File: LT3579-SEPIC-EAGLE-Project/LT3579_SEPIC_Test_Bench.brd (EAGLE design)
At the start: 74 x 58 mm, 160 parts

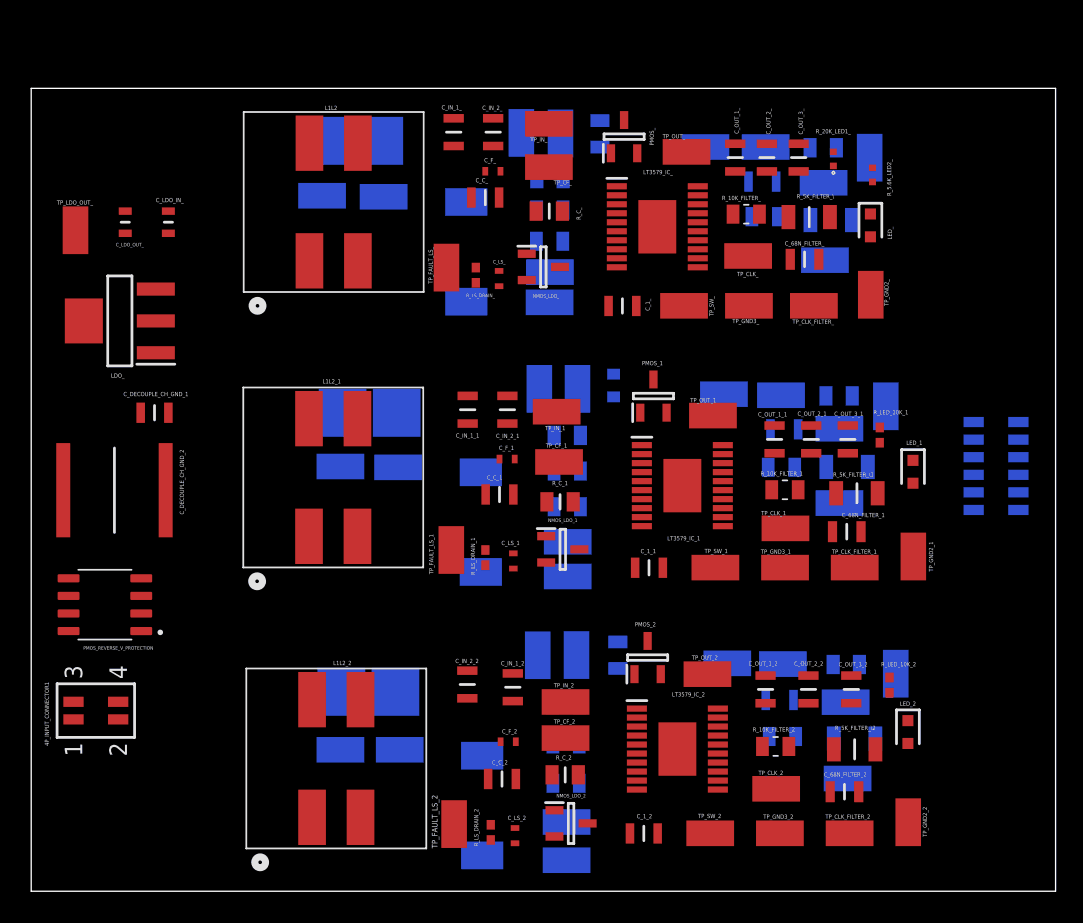
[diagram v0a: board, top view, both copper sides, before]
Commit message: Added and Replaced new files
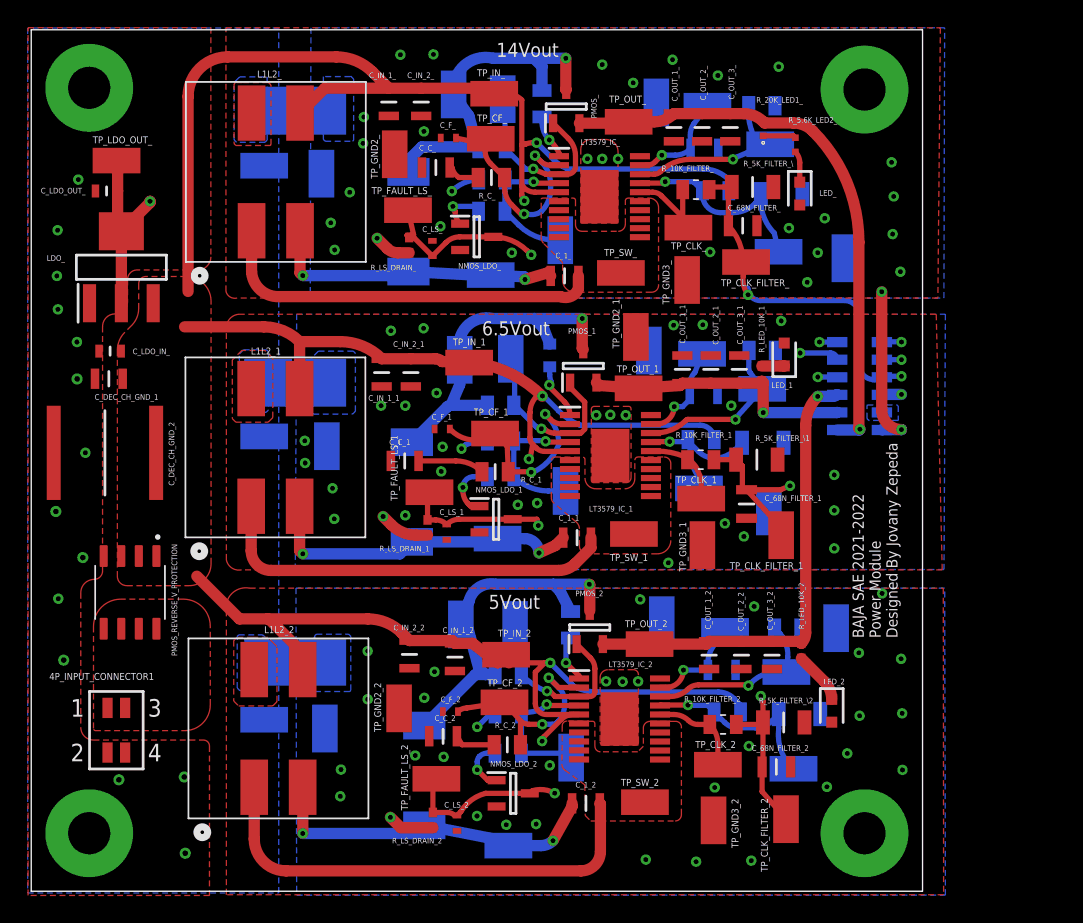
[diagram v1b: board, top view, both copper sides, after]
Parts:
- removed C_DECOUPLE_CH_GND_1: CGA4F4C0G2W222J085AE, SamacSys_Parts:CAPC2012X100N
- removed C_DECOUPLE_CH_GND_2: CGADN3X7R1E476M230LE, SamacSys_Parts:CAPC7563X250N
- added C_DEC_CH_GND_1: CGA4F4C0G2W222J085AE, SamacSys_Parts:CAPC2012X100N
- added C_DEC_CH_GND_2: CGADN3X7R1E476M230LE, SamacSys_Parts:CAPC7563X250N
- added U$1, U$2, U$3, U$4: THROUGH_HOLE_, THROUGH_HOLE:THROUGH_HOLE
- moved TP_GND2_2 37.7 mm to (26.6, 13.2), turned to 270 degrees
- moved TP_GND2_ 35.9 mm to (26.3, 53.2)
- moved TP_GND2_1 25.6 mm to (43.7, 40.0), turned to 90 degrees
- moved LED_1 12.6 mm to (54.4, 38.8), turned to 90 degrees
- moved 12P_OUTPUT_CONNECTOR1 11.4 mm to (59.8, 36.5)
- moved TP_GND4_1 11.4 mm to (53.3, 27.4), turned to 90 degrees
- moved C_LDO_IN_ 10.2 mm to (5.70, 39.0), turned to 180 degrees
- moved TP_SHDN_1 10.2 mm to (48.2, 29.1)
- moved R_LED_10K_1 9.61 mm to (52.8, 37.4), turned to 90 degrees
- moved C_OUT_3_1 9.34 mm to (51.1, 37.7), turned to 90 degrees
- moved C_OUT_2_1 8.84 mm to (49.1, 37.7), turned to 90 degrees
- moved C_OUT_1_1 8.36 mm to (47.0, 37.7), turned to 90 degrees
- moved R_5K_FILTER_\1 7.62 mm to (52.4, 31.2)
- moved C_68N_FILTER_1 7.51 mm to (51.7, 28.0), turned to 270 degrees
- moved TP_GND4_ 7.49 mm to (58.7, 45.7), turned to 90 degrees
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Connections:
- removed net 0: C_68N_FILTER_.2, C_68N_FILTER_1.2, C_68N_FILTER_2.2, C_C_.2, C_C_1.2, C_C_2.2, C_F_.2, C_F_1.2, C_F_2.2, C_IN_1_.2, C_IN_1_1.2, C_IN_1_2.2, C_IN_2_.2, C_IN_2_1.2, C_IN_2_2.2, C_LDO_IN_.2, C_LDO_OUT_.2, C_LS_.2, C_LS_1.2, C_LS_2.2, C_OUT_1_.2, C_OUT_1_1.2, C_OUT_1_2.2, C_OUT_2_.2, C_OUT_2_1.2, C_OUT_2_2.2, C_OUT_3_.2, C_OUT_3_1.2, C_OUT_3_2.2, C_SS_.2, C_SS_1.2, C_SS_2.2, L1L2_.4, L1L2_1.4, L1L2_2.4, LED_.2, LED_1.2, LED_2.2, LT3579_IC_.21, LT3579_IC_1.21, LT3579_IC_2.21, NMOS_LDO_.2, NMOS_LDO_1.2, NMOS_LDO_2.2, PMOS_REVERSE_V_PROTECTION.4, R_5K_FILTER_\.2, R_5K_FILTER_\1.2, R_5K_FILTER_\2.2, R_T_.2, R_T_1.2, R_T_2.2, R_UVLO2_.1, R_UVLO2_1.1, R_UVLO2_2.1, TP_GND1_.1, TP_GND1_1.1, TP_GND1_2.1, TP_GND2_.1, TP_GND2_1.1, TP_GND2_2.1, TP_GND3_.1, TP_GND3_1.1, TP_GND3_2.1, TP_GND4_.1, TP_GND4_1.1, TP_GND4_2.1
- removed net GND: 12P_OUTPUT_CONNECTOR1.10, 12P_OUTPUT_CONNECTOR1.12, 12P_OUTPUT_CONNECTOR1.8, LDO_.1, LT3579_IC_.20, LT3579_IC_1.20, LT3579_IC_2.20, R_SHUNT_GND_.2, R_SHUNT_GND_1.2, R_SHUNT_GND_2.2, TP_GND_.1, TP_GND_1.1, TP_GND_2.1
- new net GND_: 12P_OUTPUT_CONNECTOR1.12, C_68N_FILTER_.2, C_C_.2, C_F_.2, C_IN_1_.2, C_IN_2_.2, C_LS_.2, C_OUT_1_.2, C_OUT_2_.2, C_OUT_3_.2, C_SS_.2, L1L2_.4, LED_.2, LT3579_IC_.20, LT3579_IC_.21, NMOS_LDO_.2, R_5K_FILTER_\.2, R_SHUNT_GND_.2, R_T_.2, R_UVLO2_.1, TP_GND1_.1, TP_GND2_.1, TP_GND3_.1, TP_GND4_.1, TP_GND_.1
- new net GND_1: 12P_OUTPUT_CONNECTOR1.10, C_68N_FILTER_1.2, C_C_1.2, C_F_1.2, C_IN_1_1.2, C_IN_2_1.2, C_LS_1.2, C_OUT_1_1.2, C_OUT_2_1.2, C_OUT_3_1.2, C_SS_1.2, L1L2_1.4, LED_1.2, LT3579_IC_1.20, LT3579_IC_1.21, NMOS_LDO_1.2, R_5K_FILTER_\1.2, R_SHUNT_GND_1.2, R_T_1.2, R_UVLO2_1.1, TP_GND1_1.1, TP_GND2_1.1, TP_GND3_1.1, TP_GND4_1.1, TP_GND_1.1
- new net GND_2: 12P_OUTPUT_CONNECTOR1.8, C_68N_FILTER_2.2, C_C_2.2, C_F_2.2, C_IN_1_2.2, C_IN_2_2.2, C_LS_2.2, C_OUT_1_2.2, C_OUT_2_2.2, C_OUT_3_2.2, C_SS_2.2, L1L2_2.4, LED_2.2, LT3579_IC_2.20, LT3579_IC_2.21, NMOS_LDO_2.2, R_5K_FILTER_\2.2, R_SHUNT_GND_2.2, R_T_2.2, R_UVLO2_2.1, TP_GND1_2.1, TP_GND2_2.1, TP_GND3_2.1, TP_GND4_2.1, TP_GND_2.1
- net CH_GND: now also C_DEC_CH_GND_1.1, C_DEC_CH_GND_2.1, C_LDO_IN_.2, C_LDO_OUT_.2, LDO_.1, PMOS_REVERSE_V_PROTECTION.4; no longer C_DECOUPLE_CH_GND_1.1, C_DECOUPLE_CH_GND_2.1
- net VIN: now also C_DEC_CH_GND_1.2, C_DEC_CH_GND_2.2; no longer C_DECOUPLE_CH_GND_1.2, C_DECOUPLE_CH_GND_2.2
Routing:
- net VIN: track 0.00 -> 207.5 mm, vias 0 -> 9
- net LDO_OUT_: track 0.00 -> 92.4 mm, vias 0 -> 4
- net FAULT_LS_OUT_2: track 0.00 -> 52.5 mm, vias 0 -> 2
- net CLK_FILTER_OUT_2: track 0.00 -> 42.9 mm, vias 0 -> 2
- net VOUT_: track 0.00 -> 41.2 mm, vias 0 -> 1
- net FAULT_LS_OUT_: track 0.00 -> 37.6 mm, vias 0 -> 2
- net FAULT_LS_OUT_1: track 0.00 -> 37.0 mm, vias 0 -> 2
- net VOUT_2: track 0.00 -> 34.0 mm, vias 0 -> 1
- net SW1-2_2: track 0.00 -> 33.8 mm
- net SW1-2_1: track 0.00 -> 29.7 mm
- net SW1-2_: track 0.00 -> 28.3 mm
- net CLK_FILTER_OUT_: track 0.00 -> 26.7 mm, vias 0 -> 2
- net N$7: track 0.00 -> 26.0 mm, vias 0 -> 1
- net CLK_FILTER_OUT_1: track 0.00 -> 25.5 mm, vias 0 -> 2
- net N$3: track 0.00 -> 25.2 mm, vias 0 -> 1
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- added copper zone on layer 1, net CH_GND
- added copper zone on layer 16, net CH_GND
- added copper zone on layer 1, net GND_
- added copper zone on layer 16, net GND_
- added copper zone on layer 1, net GND_1
- added copper zone on layer 16, net GND_1
- added copper zone on layer 1, net GND_2
- added copper zone on layer 16, net GND_2
- added copper zone on layer 1, net SW1-2_
- added copper zone on layer 1, net SW1-2_1
- added copper zone on layer 1, net SW1-2_2
- added copper zone on layer 1, net VIN
- added copper zone on layer 1, net VIN_CONNECTOR
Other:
- board size 74 x 58 mm -> 64.4 x 62.2 mm
- board text added: "14Vout"
- board text added: "5Vout"
- board text added: "6.5Vout"
- board text added: "BAJA SAE 2021-2022 Power Module Designed By Jovany Zepeda"
